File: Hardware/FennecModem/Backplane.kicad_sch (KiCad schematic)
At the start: 4 parts, among them U101 NCP1117-12_SOT223

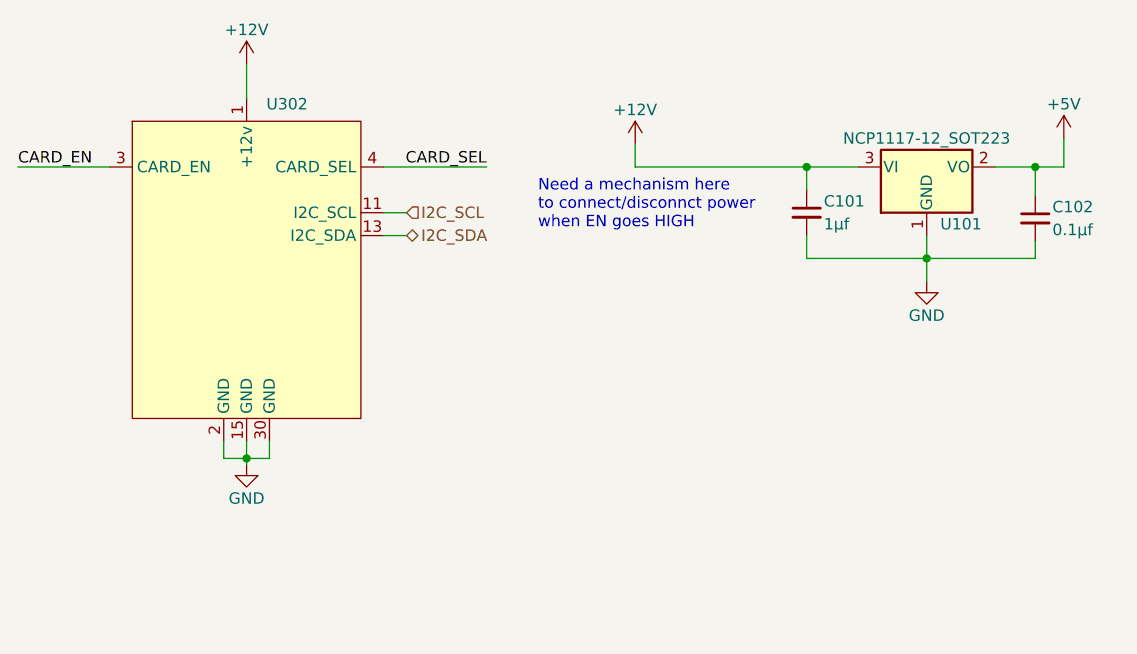
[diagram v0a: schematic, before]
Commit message: Bump backplane
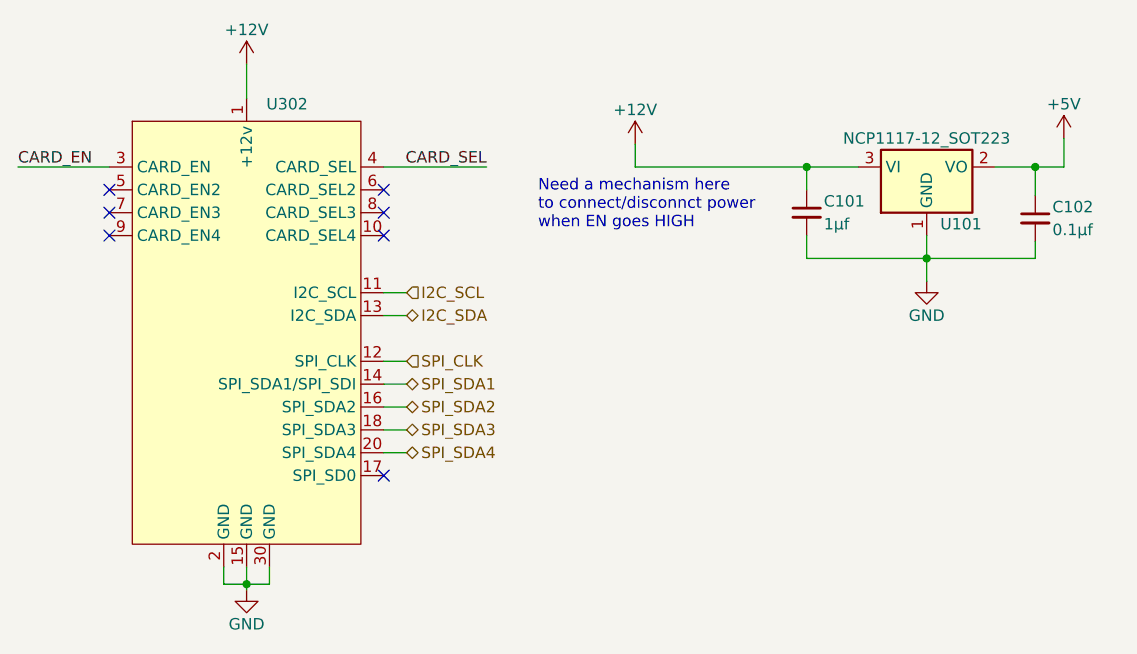
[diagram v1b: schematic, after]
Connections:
- new net SPI_CLK: U302.12 (SPI_CLK)
- new net SPI_SDA1: U302.14 (SPI_SDA1/SPI_SDI)
- new net SPI_SDA2: U302.16 (SPI_SDA2)
- new net SPI_SDA3: U302.18 (SPI_SDA3)
- new net SPI_SDA4: U302.20 (SPI_SDA4)
- no-connect marks 0 -> 7
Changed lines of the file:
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@@
   (junction (at 159.385 88.265) (diameter 0) (color 0 0 0 0)
   )
-  (junction (at 97.155 120.65) (diameter 0) (color 0 0 0 0)
+  (junction (at 97.155 134.62) (diameter 0) (color 0 0 0 0)
   )
   (junction (at 172.72 98.425) (diameter 0) (color 0 0 0 0)
   )
-  (wire (pts (xy 97.155 118.745) (xy 97.155 120.65))
+  (no_connect (at 112.395 122.555))
+  (no_connect (at 112.395 90.805))
+  (no_connect (at 81.915 95.885))
+  (no_connect (at 112.395 93.345))
+  (no_connect (at 81.915 93.345))
+  (no_connect (at 112.395 95.885))
+  (no_connect (at 81.915 90.805))
+  (wire (pts (xy 97.155 132.715) (xy 97.155 134.62))
     (stroke (width 0) (type default))
   )
@@
     (stroke (width 0) (type default))
   )
-  (wire (pts (xy 112.395 93.345) (xy 114.935 93.345))
-    (stroke (width 0) (type default))
-  )
   (wire (pts (xy 159.385 88.265) (xy 159.385 90.805))
     (stroke (width 0) (type default))
   )
-  (wire (pts (xy 99.695 120.65) (xy 99.695 118.745))
+  (wire (pts (xy 112.395 114.935) (xy 114.935 114.935))
+    (stroke (width 0) (type default))
+  )
+  (wire (pts (xy 99.695 134.62) (xy 99.695 132.715))
     (stroke (width 0) (type default))
   )
@@
     (stroke (width 0) (type default))
   )
-  (wire (pts (xy 97.155 120.65) (xy 94.615 120.65))
+  (wire (pts (xy 97.155 134.62) (xy 94.615 134.62))
     (stroke (width 0) (type default))
   )
@@
     (stroke (width 0) (type default))
   )
+  (wire (pts (xy 112.395 102.235) (xy 114.935 102.235))
+    (stroke (width 0) (type default))
+  )
+  (wire (pts (xy 112.395 120.015) (xy 114.935 120.015))
+    (stroke (width 0) (type default))
+  )
   (wire (pts (xy 97.155 76.835) (xy 97.155 80.645))
     (stroke (width 0) (type default))
@@
     (stroke (width 0) (type default))
   )
+  (wire (pts (xy 112.395 104.775) (xy 114.935 104.775))
+    (stroke (width 0) (type default))
+  )
   (wire (pts (xy 140.335 88.265) (xy 159.385 88.265))
     (stroke (width 0) (type default))
   )
-  (wire (pts (xy 112.395 95.885) (xy 114.935 95.885))
-    (stroke (width 0) (type default))
-  )
-  (wire (pts (xy 97.155 120.65) (xy 99.695 120.65))
-    (stroke (width 0) (type default))
-  )
-  (wire (pts (xy 97.155 121.285) (xy 97.155 120.65))
+  (wire (pts (xy 112.395 117.475) (xy 114.935 117.475))
+    (stroke (width 0) (type default))
+  )
+  (wire (pts (xy 112.395 112.395) (xy 114.935 112.395))
+    (stroke (width 0) (type default))
+  )
+  (wire (pts (xy 97.155 134.62) (xy 99.695 134.62))
+    (stroke (width 0) (type default))
+  )
+  (wire (pts (xy 97.155 135.255) (xy 97.155 134.62))
     (stroke (width 0) (type default))
   )
@@
     (stroke (width 0) (type default))
   )
+  (wire (pts (xy 112.395 109.855) (xy 114.935 109.855))
+    (stroke (width 0) (type default))
+  )
   (wire (pts (xy 172.72 98.425) (xy 184.785 98.425))
     (stroke (width 0) (type default))
   )
-  (wire (pts (xy 94.615 118.745) (xy 94.615 120.65))
+  (wire (pts (xy 94.615 132.715) (xy 94.615 134.62))
     (stroke (width 0) (type default))
   )
@@
     (effects (font (size 1.27 1.27)) (justify right bottom))
   )
-  (hierarchical_label "I2C_SCL" (shape input) (at 114.935 93.345 0) (fields_autoplaced)
-    (effects (font (size 1.27 1.27)) (justify left))
-  )
-  (hierarchical_label "I2C_SDA" (shape bidirectional) (at 114.935 95.885 0) (fields_autoplaced)
+  (hierarchical_label "SPI_SDA3" (shape bidirectional) (at 114.935 117.475 0) (fields_autoplaced)
+    (effects (font (size 1.27 1.27)) (justify left))
+  )
+  (hierarchical_label "SPI_SDA2" (shape bidirectional) (at 114.935 114.935 0) (fields_autoplaced)
+    (effects (font (size 1.27 1.27)) (justify left))
+  )
+  (hierarchical_label "SPI_SDA1" (shape bidirectional) (at 114.935 112.395 0) (fields_autoplaced)
+    (effects (font (size 1.27 1.27)) (justify left))
+  )
+  (hierarchical_label "SPI_SDA4" (shape bidirectional) (at 114.935 120.015 0) (fields_autoplaced)
+    (effects (font (size 1.27 1.27)) (justify left))
+  )
+  (hierarchical_label "I2C_SDA" (shape bidirectional) (at 114.935 104.775 0) (fields_autoplaced)
+    (effects (font (size 1.27 1.27)) (justify left))
+  )
+  (hierarchical_label "SPI_CLK" (shape input) (at 114.935 109.855 0) (fields_autoplaced)
+    (effects (font (size 1.27 1.27)) (justify left))
+  )
+  (hierarchical_label "I2C_SCL" (shape input) (at 114.935 102.235 0) (fields_autoplaced)
     (effects (font (size 1.27 1.27)) (justify left))
   )
@@
     )
   )
-  (symbol (lib_id "power:GND") (at 97.155 121.285 0) (unit 1)
+  (symbol (lib_id "power:GND") (at 97.155 135.255 0) (unit 1)
     (in_bom yes) (on_board yes) (dnp no)
-    (property "Reference" "#PWR0116" (at 97.155 127.635 0)
-      (effects (font (size 1.27 1.27)) hide)
-    )
-    (property "Value" "GND" (at 97.155 125.095 0)
+    (property "Reference" "#PWR0116" (at 97.155 141.605 0)
+      (effects (font (size 1.27 1.27)) hide)
+    )
+    (property "Value" "GND" (at 97.155 139.065 0)
       (effects (font (size 1.27 1.27)))
     )
-    (property "Footprint" "" (at 97.155 121.285 0)
-      (effects (font (size 1.27 1.27)) hide)
-    )
-    (property "Datasheet" "" (at 97.155 121.285 0)
+    (property "Footprint" "" (at 97.155 135.255 0)
+      (effects (font (size 1.27 1.27)) hide)
+    )
+    (property "Datasheet" "" (at 97.155 135.255 0)
       (effects (font (size 1.27 1.27)) hide)
     )
@@
     )
     (pin "1")
+    (pin "10")
     (pin "11")
+    (pin "12")
     (pin "13")
+    (pin "14")
     (pin "15")
+    (pin "16")
+    (pin "17")
+    (pin "18")
     (pin "2")
+    (pin "20")
     (pin "3")
     (pin "30")
     (pin "4")
+    (pin "5")
+    (pin "6")
+    (pin "7")
+    (pin "8")
+    (pin "9")
     (instances
       (project "FennecModem"
